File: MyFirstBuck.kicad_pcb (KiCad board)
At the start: 2 copper layers, 130.3 x 127 mm, 44 parts, among them J1 Conn_01x01_Pin, J2 Conn_01x01_Pin, J3 Conn_01x01_Pin, J4 Conn_01x01_Pin, J5 Conn_01x01_Pin, Q1 IRF540N, U1 LM358, U2 LAUNCHXL-F28379D, U3 UCC5304DWVR, U4 TMV 0512SHI

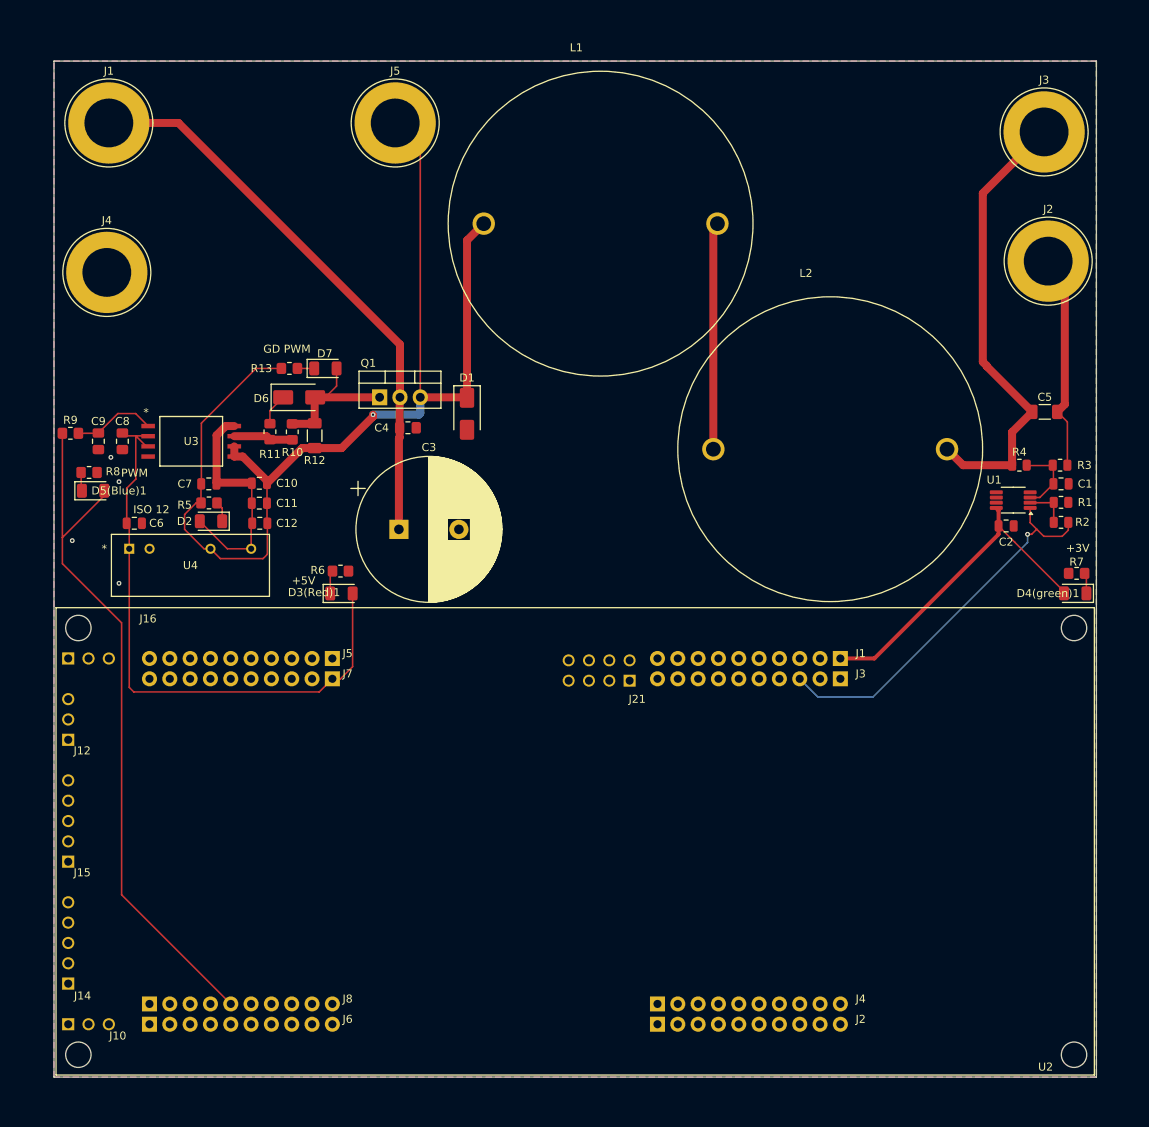
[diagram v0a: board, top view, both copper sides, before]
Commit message: Gerber and drill added
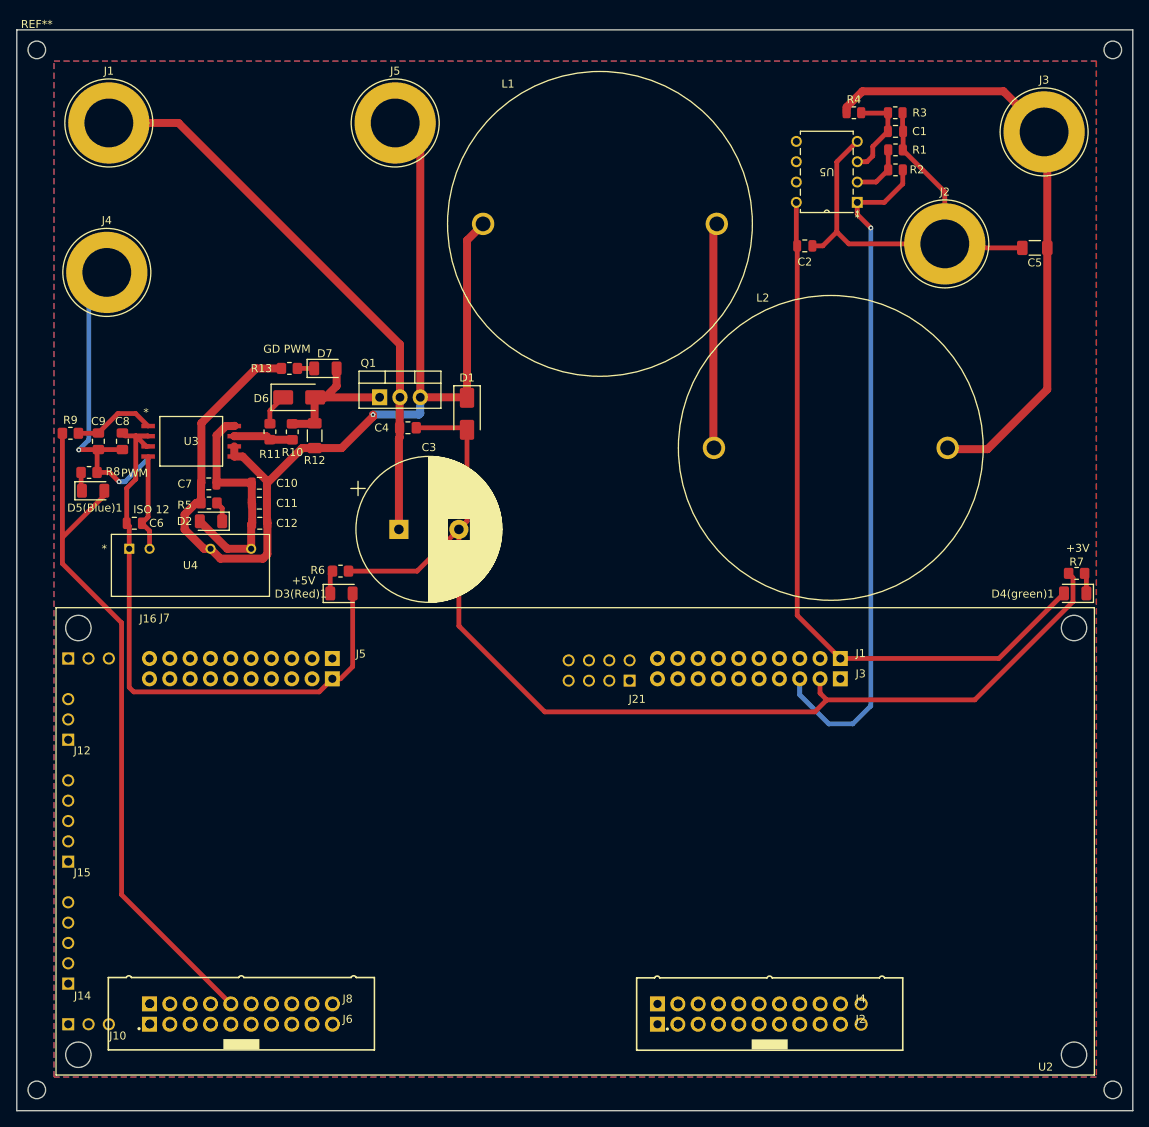
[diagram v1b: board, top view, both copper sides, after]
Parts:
- removed U1: LM358, Package_SO:VSSOP-8_3x3mm_P0.65mm
- added REF**: 61202021621, 61202021621:61202021621, F.Cu at (162.4, 144.5)
- added REF**: MountingHole_2.2mm_M2, MountingHole:MountingHole_2.2mm_M2, F.Cu at (205.2, 24.0)
- added REF**: MountingHole_2.2mm_M2, MountingHole:MountingHole_2.2mm_M2, F.Cu at (70.8, 24.0)
- added REF**: 61202021621, 61202021621:61202021621, F.Cu at (96.3, 144.5)
- added REF**: MountingHole_2.2mm_M2, MountingHole:MountingHole_2.2mm_M2, F.Cu at (70.8, 154.0)
- added REF**: MountingHole_2.2mm_M2, MountingHole:MountingHole_2.2mm_M2, F.Cu at (205.2, 154.0)
- added U5: LM358AP, LM358AP:P8, F.Cu at (165.7, 35.4)
- moved R1 48.7 mm to (178.1, 36.5)
- moved R2 48.7 mm to (178.1, 39.0)
- moved C1 48.7 mm to (178.1, 34.2)
- moved R4 48.7 mm to (172.9, 31.9)
- moved R3 48.6 mm to (178.1, 31.9)
- moved C2 43.1 mm to (166.8, 48.5)
- moved C5 20.5 mm to (195.5, 48.8), turned to 180 degrees
- moved J2 13.1 mm to (184.2, 48.2)
- moved L2 0.18 mm to (170.0, 73.8)
- moved L1 0.08 mm to (141.1, 45.8)
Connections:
- L1 pad 1: (no net) -> /VSW
- L1 pad 2: (no net) -> Net-(L1-Pad2)
- L2 pad 1: (no net) -> Net-(L1-Pad2)
- L2 pad 2: (no net) -> /VOUT
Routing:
- net GND: track 27.3 -> 252.5 mm, vias 4 -> 2
- net +3.3V: track 41.4 -> 90.6 mm
- net /VFILT: track 48.5 -> 85.4 mm
- net Net-(L1-Pad2): track 0.00 -> 28.4 mm
- net (no net): track 28.4 -> 0.00 mm
- net /VOUT: track 57.4 -> 76.3 mm
- net Net-(U5-1IN+): track 9.06 -> 11.5 mm
- net Net-(U5-1IN-): track 5.47 -> 7.06 mm
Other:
- board size 130.3 x 127 mm -> 139.5 x 135.1 mm
